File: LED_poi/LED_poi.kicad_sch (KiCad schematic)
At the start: 3 parts, among them J1 AVR-ISP-6, J2 Conn_01x02, U1 ATtiny85-20M

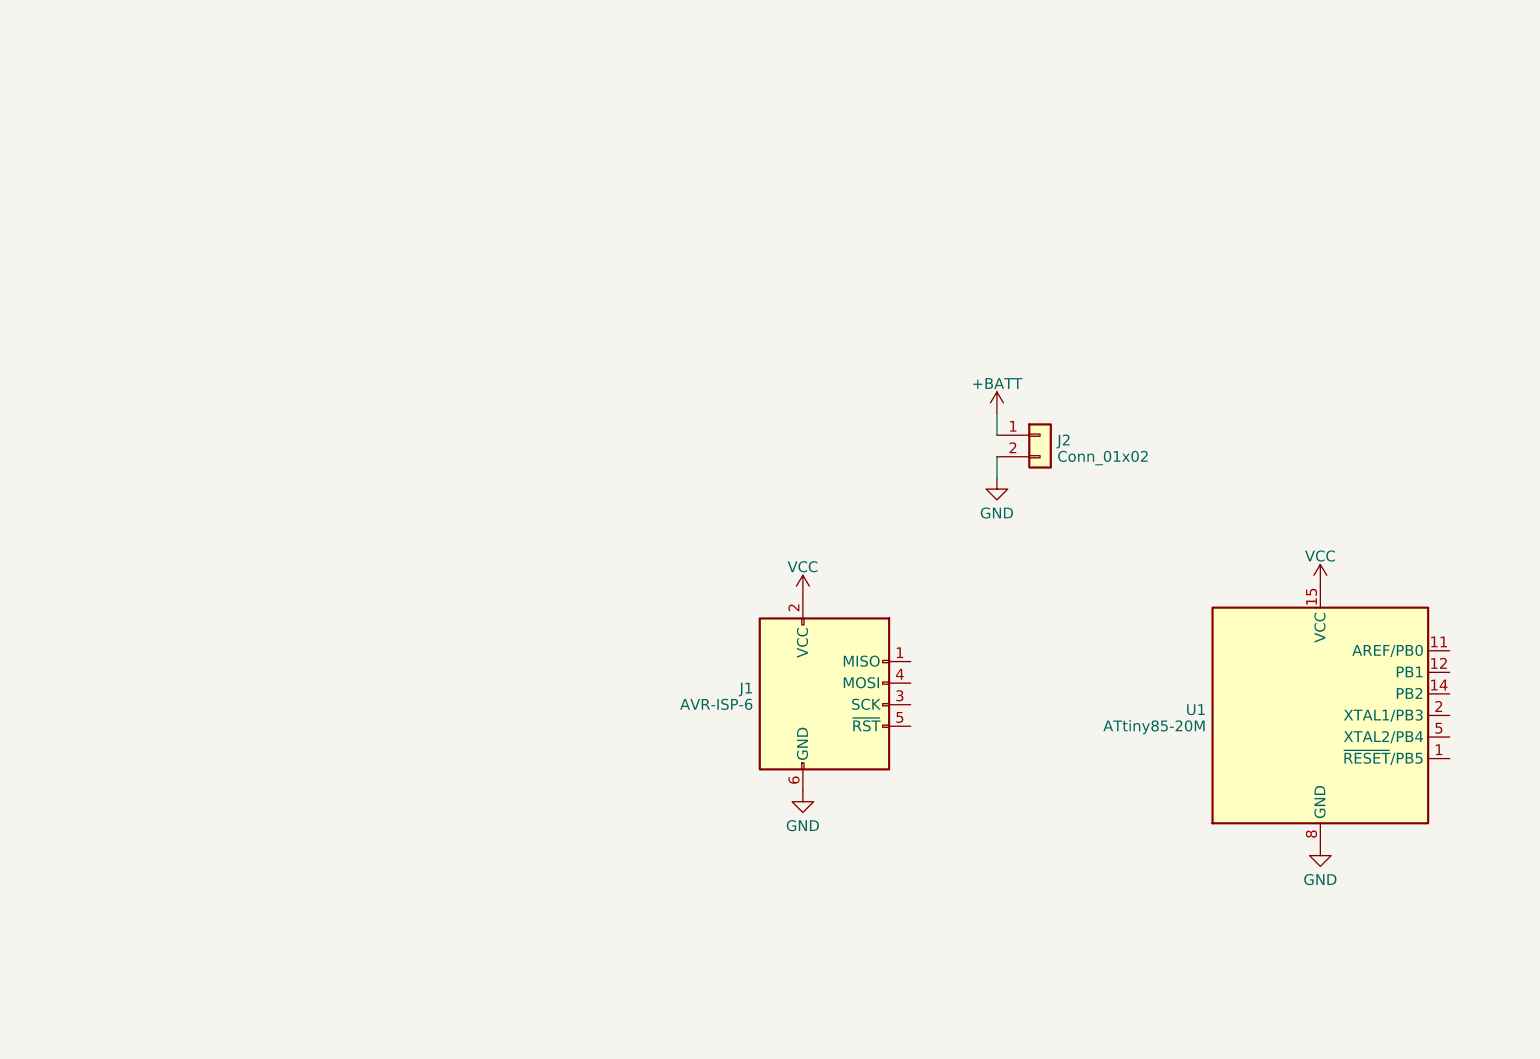
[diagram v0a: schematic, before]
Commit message: a
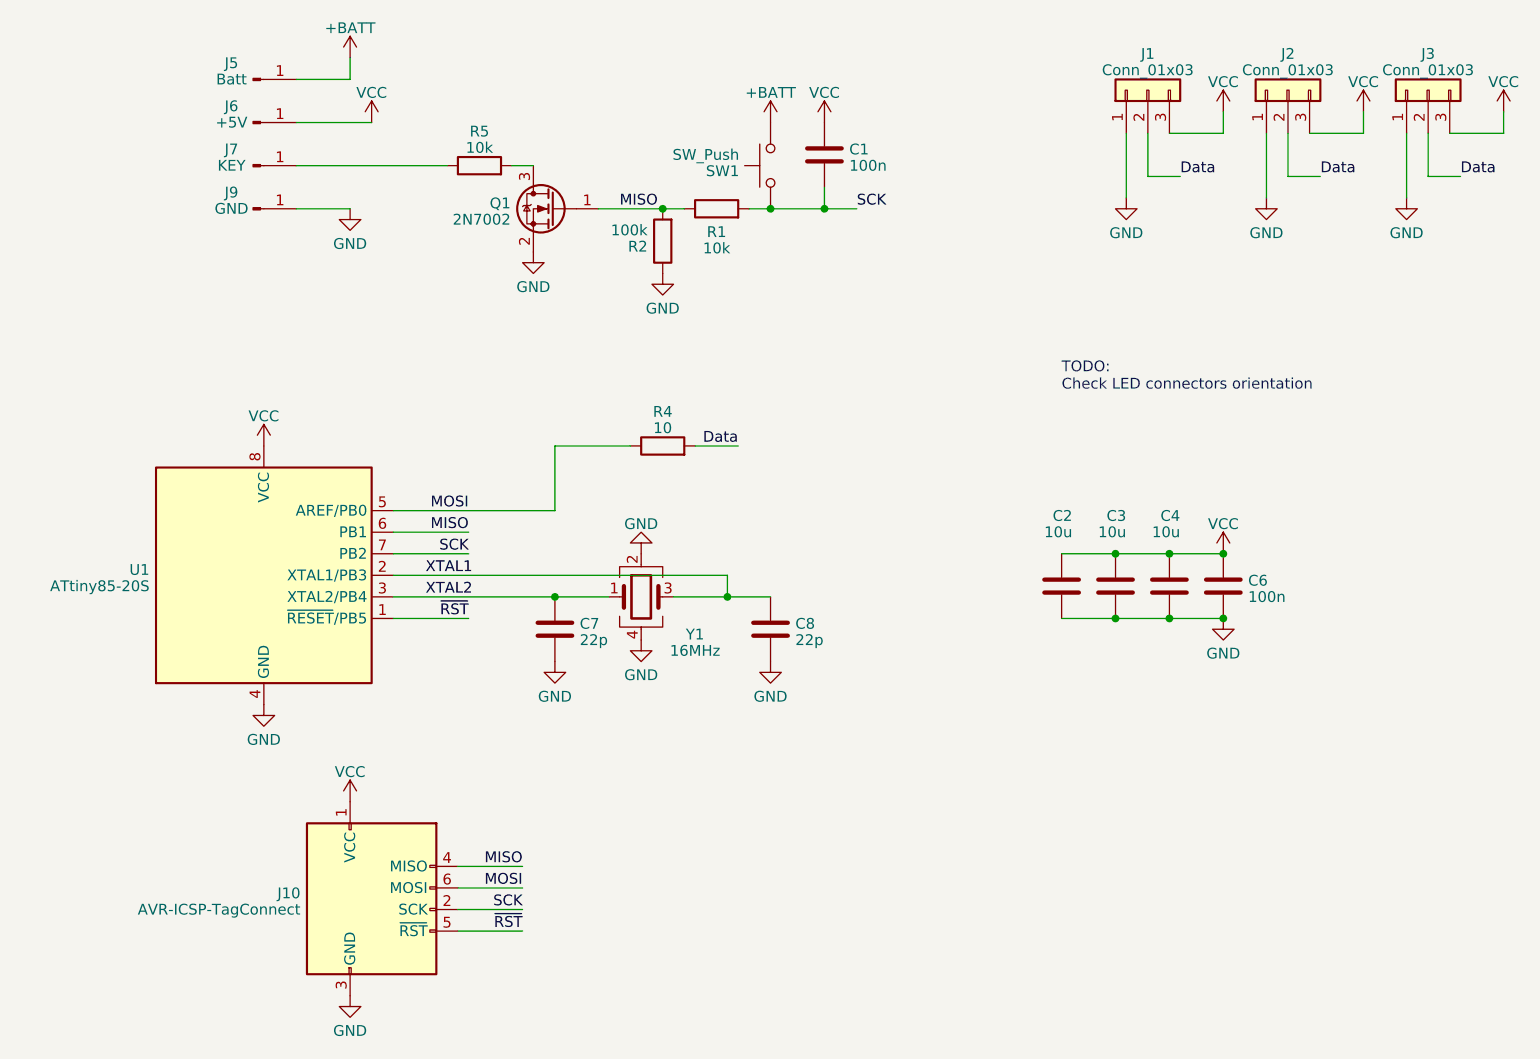
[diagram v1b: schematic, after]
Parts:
- removed J1: AVR-ISP-6, symbol Connector:AVR-ISP-6
- removed J2: Conn_01x02, symbol Connector_Generic:Conn_01x02
- removed U1: ATtiny85-20M, Package_DFN_QFN:QFN-20-1EP_4x4mm_P0.5mm_EP2.6x2.6mm, symbol MCU_Microchip_ATtiny:ATtiny85-20M
- added C1, C6: 100n, Capacitor_SMD:C_0603_1608Metric, symbol Device:C
- added C2, C3, C4: 10u, Capacitor_SMD:C_0805_2012Metric, symbol Device:C
- added C7, C8: 22p, Capacitor_SMD:C_0603_1608Metric, symbol Device:C
- added J1, J2, J3: Conn_01x03, Connector_PinHeader_2.54mm:PinHeader_1x03_P2.54mm_Vertical, symbol Connector_Generic:Conn_01x03
- added J10: AVR-ICSP-TagConnect, Connector:Tag-Connect_TC2030-IDC-NL_2x03_P1.27mm_Vertical, symbol _MYLIBRARY:AVR-ICSP-Tagconnect
- added J5: Batt, Connector_Wire:SolderWire-0.75sqmm_1x01_D1.25mm_OD2.3mm, symbol Connector:Conn_01x01_Pin
- added J6: +5V, Connector_Wire:SolderWire-0.75sqmm_1x01_D1.25mm_OD2.3mm, symbol Connector:Conn_01x01_Pin
- added J7: KEY, Connector_Wire:SolderWire-0.75sqmm_1x01_D1.25mm_OD2.3mm, symbol Connector:Conn_01x01_Pin
- added J9: GND, Connector_Wire:SolderWire-0.75sqmm_1x01_D1.25mm_OD2.3mm, symbol Connector:Conn_01x01_Pin
- added Q1: 2N7002, Package_TO_SOT_SMD:SOT-23, symbol Transistor_FET:2N7002
- added R1, R5: 10k, Resistor_SMD:R_0805_2012Metric, symbol Device:R
- added R2: 100k, Resistor_SMD:R_0805_2012Metric, symbol Device:R
- added R4: 10, Resistor_SMD:R_0805_2012Metric, symbol Device:R
- added SW1: SW_Push, footprints:TL3330, symbol Switch:SW_Push
- added U1: ATtiny85-20S, Package_SO:SOIC-8W_5.3x5.3mm_P1.27mm, symbol MCU_Microchip_ATtiny:ATtiny85-20S
- added Y1: 16MHz, Crystal:Crystal_SMD_SeikoEpson_FA238-4Pin_3.2x2.5mm_HandSoldering, symbol Device:Crystal_GND24
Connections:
- net +BATT: now also J5.1 (Pin_1), SW1.2
- net GND: now also C2.2, C3.2, C4.2, C6.2, C7.2, C8.2, J1.1 (Pin_1), J10.3 (GND), J2.1 (Pin_1), J3.1 (Pin_1), J9.1 (Pin_1), Q1.2 (S), R2.1, U1.4 (GND), Y1.2, Y1.4
- net VCC: now also C1.2, C2.1, C3.1, C4.1, C6.1, J1.3 (Pin_3), J10.1 (VCC), J2.3 (Pin_3), J3.3 (Pin_3), J6.1 (Pin_1), U1.8 (VCC)
- new net: J7.1 (Pin_1), R5.1
- new net: Q1.3 (D), R5.2
- new net Data: J1.2 (Pin_2), J2.2 (Pin_2), J3.2 (Pin_2), R4.2
- new net MISO: J10.4 (MISO), Q1.1 (G), R1.1, R2.2, U1.6 (PB1)
- new net MOSI: J10.6 (MOSI), R4.1, U1.5 (AREF/PB0)
- new net SCK: C1.1, J10.2 (SCK), R1.2, SW1.1, U1.7 (PB2)
- new net XTAL1: C8.1, U1.2 (XTAL1/PB3), Y1.3
- new net XTAL2: C7.1, U1.3 (XTAL2/PB4), Y1.1
- new net ~{RST}: J10.5 (~{RST}), U1.1 (~{RESET}/PB5)
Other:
- note added: "TODO: Check LED connectors orientation"
- company: (none) -> Author: X.B.
- title: (none) -> LED Poi driver

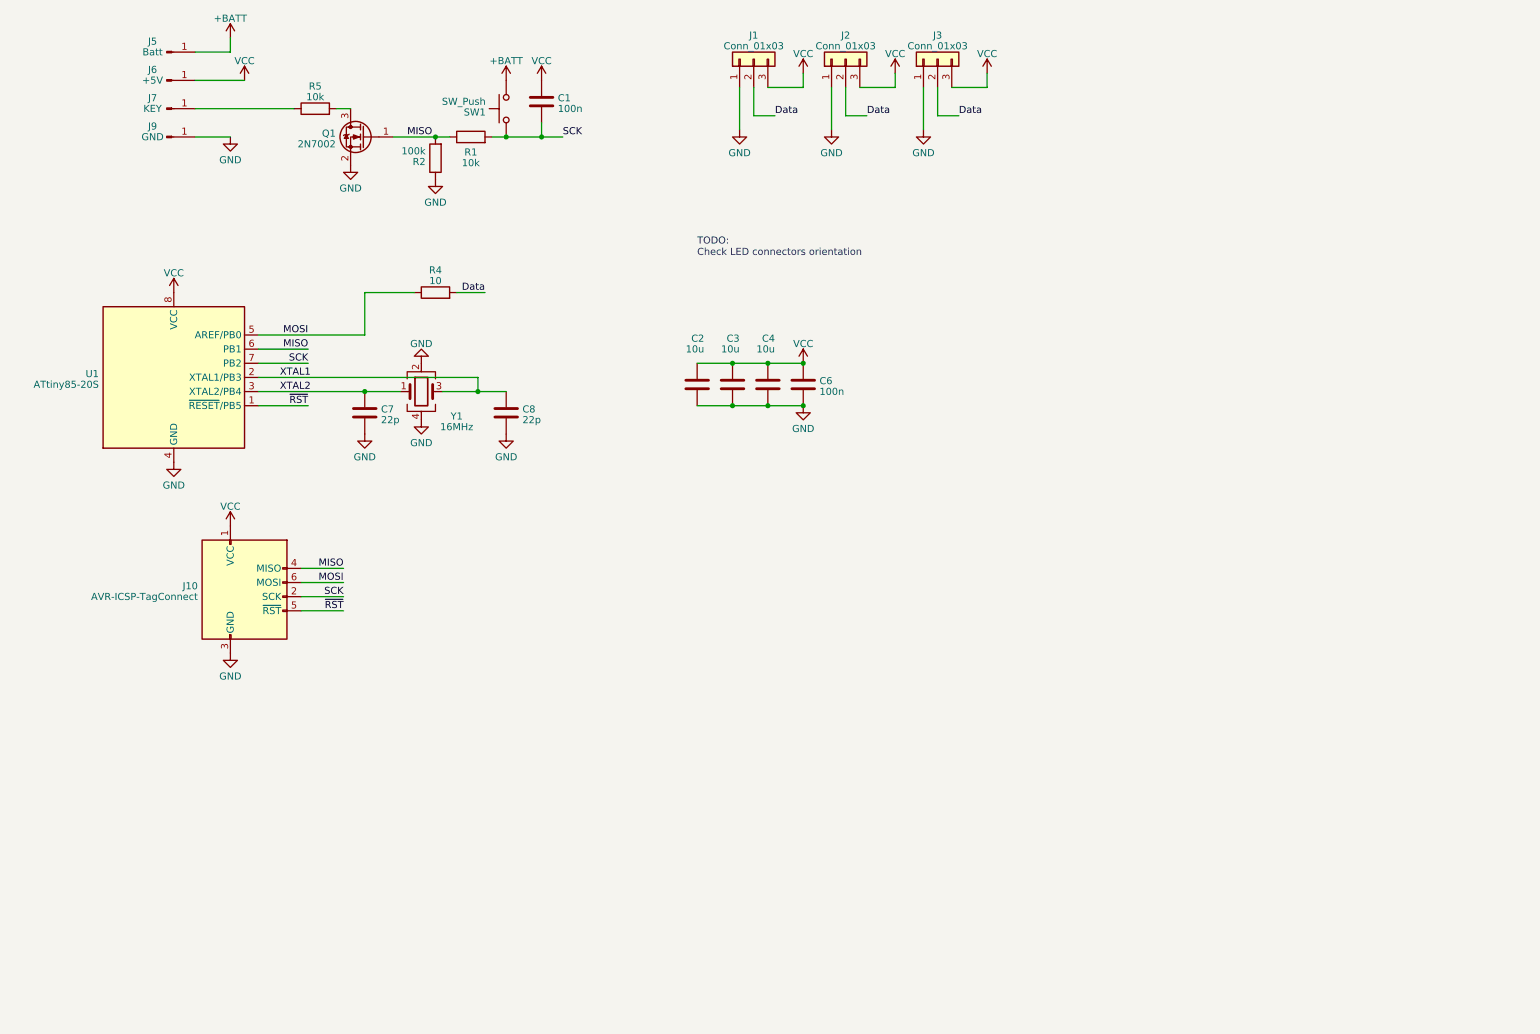
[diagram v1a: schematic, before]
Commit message: a
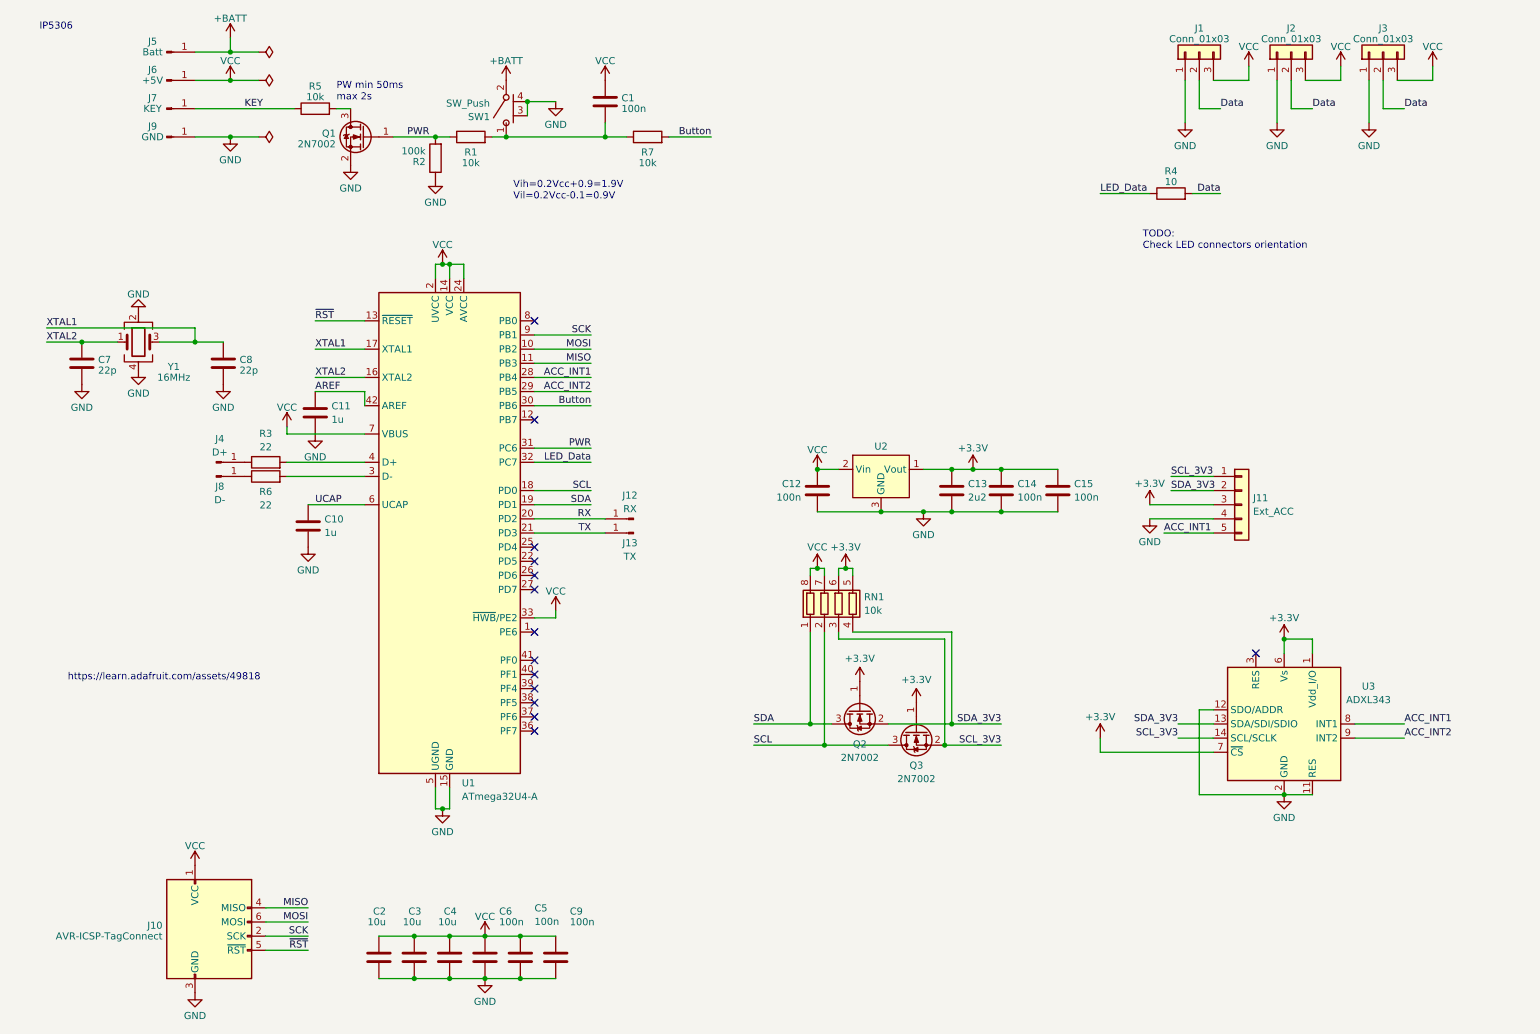
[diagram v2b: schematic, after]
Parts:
- removed U1: ATtiny85-20S, Package_SO:SOIC-8W_5.3x5.3mm_P1.27mm, symbol MCU_Microchip_ATtiny:ATtiny85-20S
- added C10, C11: 1u, Capacitor_SMD:C_0603_1608Metric, symbol Device:C
- added C12, C14, C15, C5, C9: 100n, Capacitor_SMD:C_0603_1608Metric, symbol Device:C
- added C13: 2u2, Capacitor_SMD:C_0603_1608Metric, symbol Device:C
- added J11: Ext_ACC, Connector_PinHeader_2.54mm:PinHeader_1x05_P2.54mm_Vertical, symbol Connector_Generic:Conn_01x05
- added J12: RX, Connector_Wire:SolderWirePad_1x01_SMD_1x2mm, symbol Connector:Conn_01x01_Pin
- added J13: TX, Connector_Wire:SolderWirePad_1x01_SMD_1x2mm, symbol Connector:Conn_01x01_Pin
- added J4: D+, Connector_Wire:SolderWire-0.1sqmm_1x01_D0.4mm_OD1mm, symbol Connector:Conn_01x01_Pin
- added J8: D-, Connector_Wire:SolderWire-0.1sqmm_1x01_D0.4mm_OD1mm, symbol Connector:Conn_01x01_Pin
- added Q2, Q3: 2N7002, Package_TO_SOT_SMD:SOT-23, symbol Transistor_FET:2N7002
- added R3, R6: 22, Resistor_SMD:R_0805_2012Metric, symbol Device:R
- added R7: 10k, Resistor_SMD:R_0805_2012Metric, symbol Device:R
- added RN1: 10k, Resistor_SMD:R_Array_Convex_4x1206, symbol Device:R_Pack04
- added U1: ATmega32U4-A, Package_QFP:TQFP-44_10x10mm_P0.8mm, symbol MCU_Microchip_ATmega:ATmega32U4-A
- added U2: ~, Package_TO_SOT_SMD:SOT-23, symbol _MYLIBRARY:MCP1810T-33I/TT
- added U3: ADXL343, Package_LGA:LGA-14_3x5mm_P0.8mm_LayoutBorder1x6y, symbol Sensor_Motion:ADXL343
- J1, J10, J2, J3, J5, J6, J9: DNP (none) -> x
- J7: footprint Connector_Wire:SolderWire-0.75sqmm_1x01_D1.25mm_OD2.3mm -> Connector_Wire:SolderWire-0.1sqmm_1x01_D0.4mm_OD1mm; DNP (none) -> x
- SW1: symbol Switch:SW_Push -> _MYLIBRARY:SW_SPDT_shield_1
- Y1: footprint Crystal:Crystal_SMD_SeikoEpson_FA238-4Pin_3.2x2.5mm_HandSoldering -> Crystal:Crystal_SMD_SeikoEpson_FA238-4Pin_3.2x2.5mm
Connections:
- net GND: now also SW1.3 (C), SW1.4 (Shield), C10.2, C11.2, C12.2, C13.2, C14.2, C15.2, C5.2, C9.2, J11.4 (Pin_4), U1.15 (GND), U1.23 (GND), U1.35 (GND), U1.43 (GND), U1.5 (UGND), U2.3 (GND), U3.11 (RES), U3.12 (SDO/ADDR), U3.2 (GND), U3.4 (GND), U3.5 (GND)
- net MISO: now also U1.11 (PB3); no longer Q1.1 (G), R1.1, R2.2
- net MOSI: now also U1.10 (PB2); no longer R4.1
- net SCK: now also U1.9 (PB1); no longer C1.1, R1.2, SW1.1
- net VCC: now also C12.1, C5.1, C9.1, RN1.7 (R2.2), RN1.8 (R1.2), U1.14 (VCC), U1.2 (UVCC), U1.24 (AVCC), U1.33 (~{HWB}/PE2), U1.34 (VCC), U1.44 (AVCC), U1.7 (VBUS), U2.2 (Vin)
- net XTAL1: now also U1.17 (XTAL1)
- net XTAL2: now also U1.16 (XTAL2)
- net ~{RST}: now also U1.13 (~{RESET})
- net KEY: now reaches J7.1 (Pin_1), R5.1
- new net: C1.1, R1.2, R7.1, SW1.1 (A)
- new net: J4.1 (Pin_1), R3.1
- new net: R3.2, U1.4 (D+)
- new net: R6.2, U1.3 (D-)
- new net: J8.1 (Pin_1), R6.1
- new net +3.3V: C13.1, C14.1, C15.1, J11.3 (Pin_3), Q2.1 (G), Q3.1 (G), RN1.5 (R4.2), RN1.6 (R3.2), U2.1 (Vout), U3.1 (Vdd_I/O), U3.6 (Vs), U3.7 (~{CS})
- new net ACC_INT1: J11.5 (Pin_5), U1.28 (PB4), U3.8 (INT1)
- new net ACC_INT2: U1.29 (PB5), U3.9 (INT2)
- new net AREF: C11.1, U1.42 (AREF)
- new net Button: R7.2, U1.30 (PB6)
- new net LED_Data: R4.1, U1.32 (PC7)
- new net PWR: Q1.1 (G), R1.1, R2.2, U1.31 (PC6)
- new net RX: J12.1 (Pin_1), U1.20 (PD2)
- new net SCL: Q3.3 (D), RN1.2 (R2.1), U1.18 (PD0)
- new net SCL_3V3: J11.1 (Pin_1), Q3.2 (S), RN1.3 (R3.1), U3.14 (SCL/SCLK)
- new net SDA: Q2.3 (D), RN1.1 (R1.1), U1.19 (PD1)
- new net SDA_3V3: J11.2 (Pin_2), Q2.2 (S), RN1.4 (R4.1), U3.13 (SDA/SDI/SDIO)
- new net TX: J13.1 (Pin_1), U1.21 (PD3)
- new net UCAP: C10.1, U1.6 (UCAP)
- no-connect marks 0 -> 14
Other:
- note added: "IP5306"
- note added: "PW min 50ms max 2s"
- note added: "Vih=0.2Vcc+0.9=1.9V Vil=0.2Vcc-0.1=0.9V"
- note added: "https://learn.adafruit.com/assets/49818"
- moved on the sheet: C1, C2, C3, C4, C6, C7, C8, J1, J10, J2, J3, R4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
